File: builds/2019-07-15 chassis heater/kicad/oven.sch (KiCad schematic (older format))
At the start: 13 parts, among them Q1 TIP122, U1 LM324

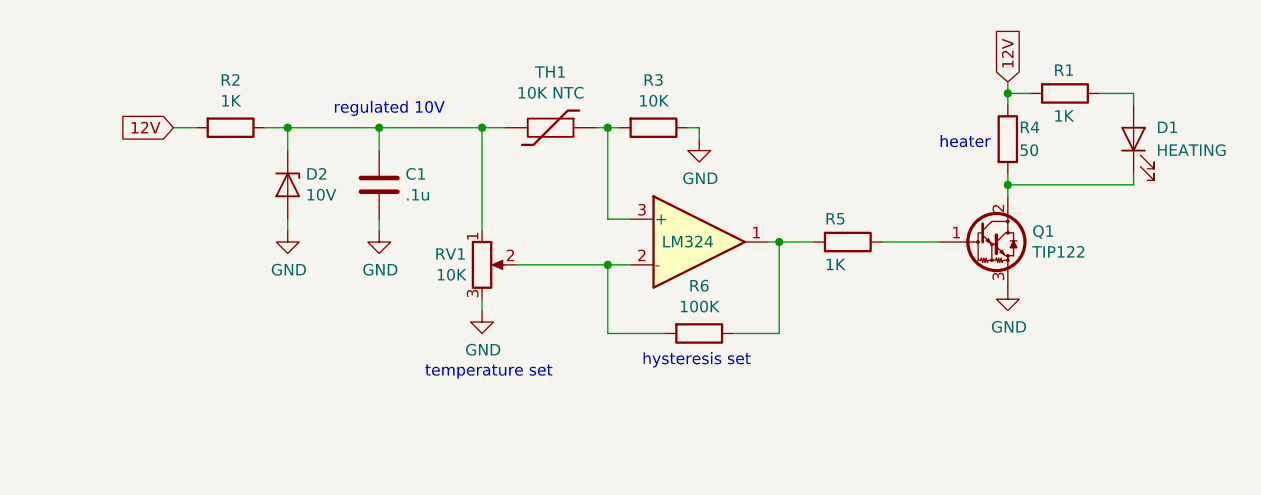
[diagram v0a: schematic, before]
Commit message: fix schematic
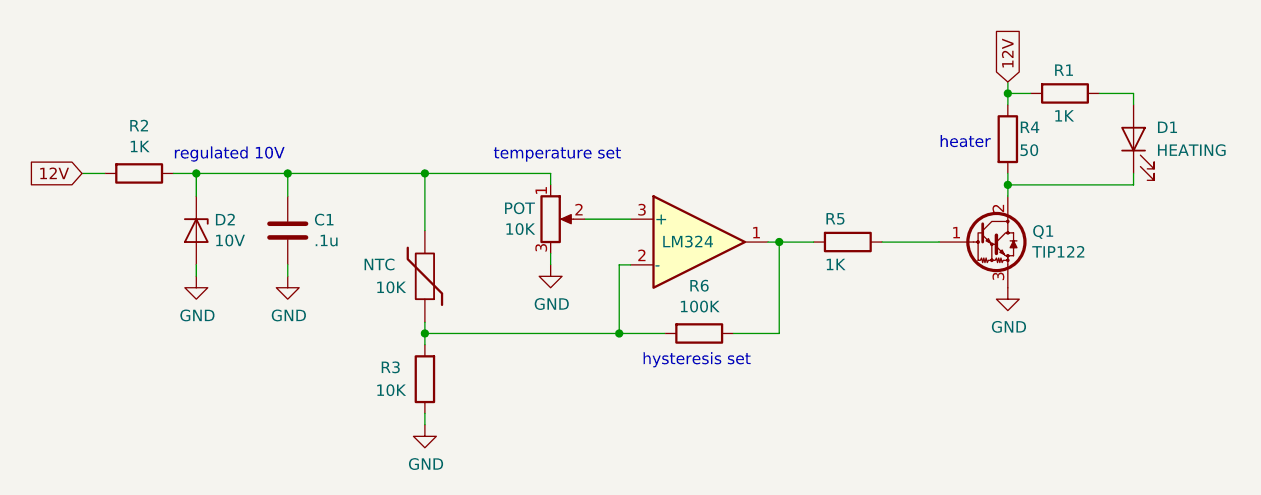
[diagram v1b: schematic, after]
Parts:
- NTC: renamed from TH1; value 10K NTC -> 10K
- renumbered RV1 to POT
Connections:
- net at R6.2, U1.2 (-): now also NTC.1, R3.2; no longer POT.2
- new net: POT.2, U1.3 (+)
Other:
- moved on the sheet: C1, D2, NTC, POT, R2, R3
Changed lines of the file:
@@
 Text Notes 4050 4800 0    50   ~ 0
 hysteresis set
-Wire Wire Line
-	4000 4350 3900 4350
 $Comp
 L power:GND #PWR04
@@
 $EndComp
 Wire Wire Line
-	4150 4650 3900 4650
-Wire Wire Line
-	3900 4350 3900 4650
-Wire Wire Line
 	4450 4650 4650 4650
 Wire Wire Line
@@
 Wire Wire Line
 	5650 3600 5650 3650
-Wire Wire Line
-	3850 3750 3900 3750
-Wire Wire Line
-	4000 4150 3900 4150
-$Comp
-L Device:Thermistor TH1
-U 1 1 5D2C2C3C
-P 3650 3750
-F 0 "TH1" V 3408 3750 50  0000 C CNN
-F 1 "10K NTC" V 3499 3750 50  0000 C CNN
-F 2 "" H 3650 3750 50  0001 C CNN
-F 3 "~" H 3650 3750 50  0001 C CNN
-	1    3650 3750
-	0    1    1    0
-$EndComp
-$Comp
-L Device:R R3
-U 1 1 5D2C3CBB
-P 4100 3750
-F 0 "R3" V 3893 3750 50  0000 C CNN
-F 1 "10K" V 3984 3750 50  0000 C CNN
-F 2 "" V 4030 3750 50  0001 C CNN
-F 3 "~" H 4100 3750 50  0001 C CNN
-	1    4100 3750
-	0    1    1    0
-$EndComp
-$Comp
-L power:GND #PWR01
-U 1 1 5D2C466F
-P 4300 3800
-F 0 "#PWR01" H 4300 3550 50  0001 C CNN
-F 1 "GND" H 4305 3627 50  0000 C CNN
-F 2 "" H 4300 3800 50  0001 C CNN
-F 3 "" H 4300 3800 50  0001 C CNN
-	1    4300 3800
-	1    0    0    -1
-$EndComp
-Wire Wire Line
-	4250 3750 4300 3750
-Wire Wire Line
-	4300 3750 4300 3800
+$Comp
+L Device:R R6
+U 1 1 5D2C751B
+P 4300 4650
+F 0 "R6" V 4093 4650 50  0000 C CNN
+F 1 "100K" V 4184 4650 50  0000 C CNN
+F 2 "" V 4230 4650 50  0001 C CNN
+F 3 "~" H 4300 4650 50  0001 C CNN
+	1    4300 4650
+	0    1    1    0
+$EndComp
+$Comp
+L power:GND #PWR05
+U 1 1 5D2C8B17
+P 3650 4350
+F 0 "#PWR05" H 3650 4100 50  0001 C CNN
+F 1 "GND" H 3655 4177 50  0000 C CNN
+F 2 "" H 3650 4350 50  0001 C CNN
+F 3 "" H 3650 4350 50  0001 C CNN
+	1    3650 4350
+	1    0    0    -1
+$EndComp
+Wire Wire Line
+	3650 4300 3650 4350
+Text Notes 5350 3850 0    50   ~ 0
+heater
+Wire Wire Line
+	2100 4350 2100 4400
+$Comp
+L power:GND #PWR02
+U 1 1 5D2CDC79
+P 2100 4400
+F 0 "#PWR02" H 2100 4150 50  0001 C CNN
+F 1 "GND" H 2105 4227 50  0000 C CNN
+F 2 "" H 2100 4400 50  0001 C CNN
+F 3 "" H 2100 4400 50  0001 C CNN
+	1    2100 4400
+	1    0    0    -1
+$EndComp
+Wire Wire Line
+	2500 4350 2500 4400
+$Comp
+L power:GND #PWR03
+U 1 1 5D2D200A
+P 2500 4400
+F 0 "#PWR03" H 2500 4150 50  0001 C CNN
+F 1 "GND" H 2505 4227 50  0000 C CNN
+F 2 "" H 2500 4400 50  0001 C CNN
+F 3 "" H 2500 4400 50  0001 C CNN
+	1    2500 4400
+	1    0    0    -1
+$EndComp
 $Comp
 L Amplifier_Operational:LM324 U1
@@
 	1    0    0    -1
 $EndComp
-Wire Wire Line
-	3900 3750 3900 4150
-Connection ~ 3900 3750
-Wire Wire Line
-	3900 3750 3950 3750
-$Comp
-L Device:R_POT RV1
-U 1 1 5D2C651A
-P 3350 4350
-F 0 "RV1" H 3281 4396 50  0000 R CNN
-F 1 "10K" H 3281 4305 50  0000 R CNN
-F 2 "" H 3350 4350 50  0001 C CNN
-F 3 "~" H 3350 4350 50  0001 C CNN
-	1    3350 4350
-	1    0    0    -1
-$EndComp
-$Comp
-L Device:R R6
-U 1 1 5D2C751B
-P 4300 4650
-F 0 "R6" V 4093 4650 50  0000 C CNN
-F 1 "100K" V 4184 4650 50  0000 C CNN
-F 2 "" V 4230 4650 50  0001 C CNN
-F 3 "~" H 4300 4650 50  0001 C CNN
-	1    4300 4650
-	0    1    1    0
-$EndComp
-Connection ~ 3900 4350
-$Comp
-L power:GND #PWR05
-U 1 1 5D2C8B17
-P 3350 4550
-F 0 "#PWR05" H 3350 4300 50  0001 C CNN
-F 1 "GND" H 3355 4377 50  0000 C CNN
-F 2 "" H 3350 4550 50  0001 C CNN
-F 3 "" H 3350 4550 50  0001 C CNN
-	1    3350 4550
-	1    0    0    -1
-$EndComp
-Wire Wire Line
-	3350 4500 3350 4550
-Wire Wire Line
-	3450 3750 3350 3750
-Wire Wire Line
-	3350 3750 3350 4200
-Wire Wire Line
-	3500 4350 3900 4350
-Text Notes 3100 4850 0    50   ~ 0
-temperature set
-Text Notes 5350 3850 0    50   ~ 0
-heater
-Wire Wire Line
-	2500 3750 2500 3850
-Wire Wire Line
-	2400 3750 2500 3750
-Wire Wire Line
-	2500 4150 2500 4200
-$Comp
-L power:GND #PWR02
-U 1 1 5D2CDC79
+Text Notes 2000 3900 0    50   ~ 0
+regulated 10V
+Connection ~ 2500 3950
+Connection ~ 2100 3950
+Wire Wire Line
+	2500 3950 2500 4050
+Wire Wire Line
+	2100 3950 2500 3950
+$Comp
+L Device:C C1
+U 1 1 5D2D0DD5
 P 2500 4200
-F 0 "#PWR02" H 2500 3950 50  0001 C CNN
-F 1 "GND" H 2505 4027 50  0000 C CNN
-F 2 "" H 2500 4200 50  0001 C CNN
-F 3 "" H 2500 4200 50  0001 C CNN
+F 0 "C1" H 2615 4246 50  0000 L CNN
+F 1 ".1u" H 2615 4155 50  0000 L CNN
+F 2 "" H 2538 4050 50  0001 C CNN
+F 3 "~" H 2500 4200 50  0001 C CNN
 	1    2500 4200
 	1    0    0    -1
 $EndComp
+Text GLabel 1600 3950 0    50   Input ~ 0
+12V
+$Comp
+L Device:R R2
+U 1 1 5D2CB7E2
+P 1850 3950
+F 0 "R2" V 1643 3950 50  0000 C CNN
+F 1 "1K" V 1734 3950 50  0000 C CNN
+F 2 "" V 1780 3950 50  0001 C CNN
+F 3 "~" H 1850 3950 50  0001 C CNN
+	1    1850 3950
+	0    1    1    0
+$EndComp
+Wire Wire Line
+	1700 3950 1600 3950
 $Comp
 L Device:D_Zener D2
 U 1 1 5D2CCC53
-P 2500 4000
-F 0 "D2" V 2454 4079 50  0000 L CNN
-F 1 "10V" V 2545 4079 50  0000 L CNN
-F 2 "" H 2500 4000 50  0001 C CNN
-F 3 "~" H 2500 4000 50  0001 C CNN
-	1    2500 4000
-	0    1    1    0
-$EndComp
-Wire Wire Line
-	2100 3750 2000 3750
-$Comp
-L Device:R R2
-U 1 1 5D2CB7E2
-P 2250 3750
-F 0 "R2" V 2043 3750 50  0000 C CNN
-F 1 "1K" V 2134 3750 50  0000 C CNN
-F 2 "" V 2180 3750 50  0001 C CNN
-F 3 "~" H 2250 3750 50  0001 C CNN
-	1    2250 3750
-	0    1    1    0
-$EndComp
-Text GLabel 2000 3750 0    50   Input ~ 0
-12V
-$Comp
-L Device:C C1
-U 1 1 5D2D0DD5
-P 2900 4000
-F 0 "C1" H 3015 4046 50  0000 L CNN
-F 1 ".1u" H 3015 3955 50  0000 L CNN
-F 2 "" H 2938 3850 50  0001 C CNN
-F 3 "~" H 2900 4000 50  0001 C CNN
-	1    2900 4000
-	1    0    0    -1
-$EndComp
-Wire Wire Line
-	2900 4150 2900 4200
-$Comp
-L power:GND #PWR03
-U 1 1 5D2D200A
-P 2900 4200
-F 0 "#PWR03" H 2900 3950 50  0001 C CNN
-F 1 "GND" H 2905 4027 50  0000 C CNN
-F 2 "" H 2900 4200 50  0001 C CNN
-F 3 "" H 2900 4200 50  0001 C CNN
-	1    2900 4200
-	1    0    0    -1
-$EndComp
-Wire Wire Line
-	2500 3750 2900 3750
-Wire Wire Line
-	2900 3750 2900 3850
-Connection ~ 2500 3750
-Wire Wire Line
-	2900 3750 3350 3750
-Connection ~ 2900 3750
-Connection ~ 3350 3750
-Text Notes 2700 3700 0    50   ~ 0
-regulated 10V
+P 2100 4200
+F 0 "D2" V 2054 4279 50  0000 L CNN
+F 1 "10V" V 2145 4279 50  0000 L CNN
+F 2 "" H 2100 4200 50  0001 C CNN
+F 3 "~" H 2100 4200 50  0001 C CNN
+	1    2100 4200
+	0    1    1    0
+$EndComp
+Wire Wire Line
+	2000 3950 2100 3950
+Wire Wire Line
+	2100 3950 2100 4050
+Wire Wire Line
+	3100 4600 3100 4650
+$Comp
+L Device:Thermistor NTC
+U 1 1 5D2C2C3C
+P 3100 4400
+F 0 "NTC" H 3300 4350 50  0000 C CNN
+F 1 "10K" H 3250 4450 50  0000 C CNN
+F 2 "" H 3100 4400 50  0001 C CNN
+F 3 "~" H 3100 4400 50  0001 C CNN
+	1    3100 4400
+	-1   0    0    1
+$EndComp
+$Comp
+L power:GND #PWR01
+U 1 1 5D2C466F
+P 3100 5050
+F 0 "#PWR01" H 3100 4800 50  0001 C CNN
+F 1 "GND" H 3105 4877 50  0000 C CNN
+F 2 "" H 3100 5050 50  0001 C CNN
+F 3 "" H 3100 5050 50  0001 C CNN
+	1    3100 5050
+	1    0    0    -1
+$EndComp
+Wire Wire Line
+	3100 5000 3100 5050
+Wire Wire Line
+	3800 4150 4000 4150
+Wire Wire Line
+	3100 4650 3950 4650
+Connection ~ 3100 4650
+Wire Wire Line
+	3100 4650 3100 4700
+$Comp
+L Device:R R3
+U 1 1 5D2C3CBB
+P 3100 4850
+F 0 "R3" H 3250 4800 50  0000 C CNN
+F 1 "10K" H 3250 4900 50  0000 C CNN
+F 2 "" V 3030 4850 50  0001 C CNN
+F 3 "~" H 3100 4850 50  0001 C CNN
+	1    3100 4850
+	-1   0    0    1
+$EndComp
+Wire Wire Line
+	3650 4000 3650 3950
+Wire Wire Line
+	3650 3950 3100 3950
+Wire Wire Line
+	3100 3950 3100 4200
+Wire Wire Line
+	2500 3950 3100 3950
+Connection ~ 3100 3950
+Wire Wire Line
+	4000 4350 3950 4350
+Wire Wire Line
+	3950 4350 3950 4650
+Connection ~ 3950 4650
+Wire Wire Line
+	3950 4650 4150 4650
+$Comp
+L Device:R_POT POT
+U 1 1 5D2C651A
+P 3650 4150
+F 0 "POT" H 3581 4196 50  0000 R CNN
+F 1 "10K" H 3581 4105 50  0000 R CNN
+F 2 "" H 3650 4150 50  0001 C CNN
+F 3 "~" H 3650 4150 50  0001 C CNN
+	1    3650 4150
+	1    0    0    -1
+$EndComp
+Text Notes 3400 3900 0    50   ~ 0
+temperature set
 $EndSCHEMATC
